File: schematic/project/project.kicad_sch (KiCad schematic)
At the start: 4 parts, among them U1 NFC IC

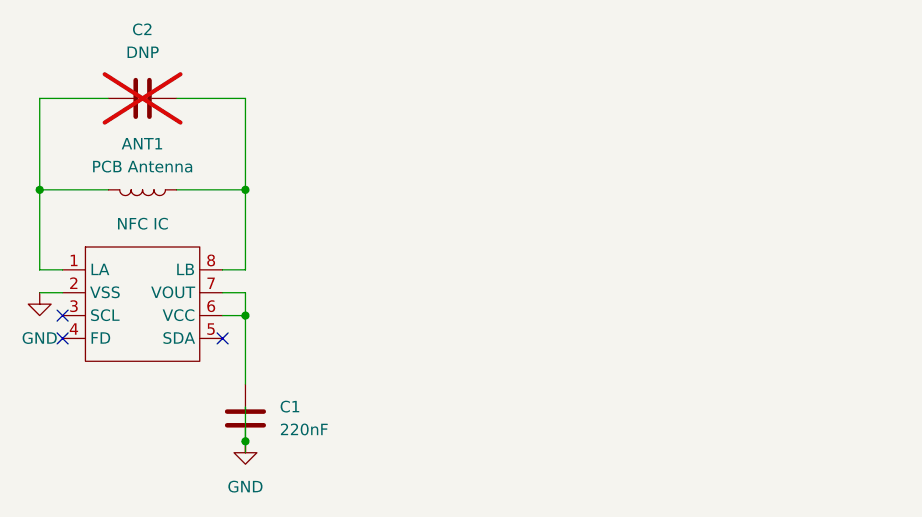
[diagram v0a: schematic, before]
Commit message: ??
After not realizing for nearly two weeks I finally committed proper workfiles with updated progress on the PCB of the card
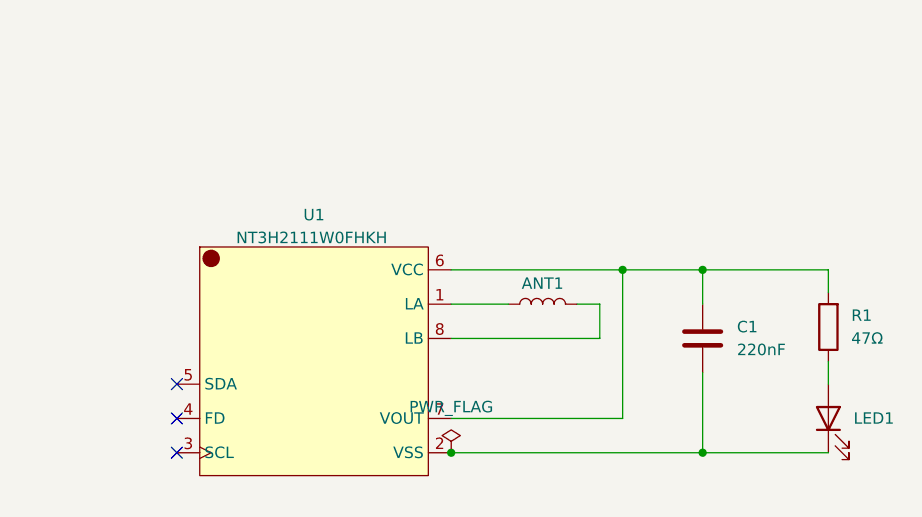
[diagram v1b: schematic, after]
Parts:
- removed C2: DNP, Capacitor_SMD:C_0805_2012Metric, symbol Device:C
- removed U1: NFC IC, Package_SO:TSSOP-8_3x3mm_P0.65mm, symbol local:NT3H2111W0FTTJ
- added LED1: LED, LED_SMD:LED_0805_2012Metric, symbol Device:LED
- added R1: 47Ω, Resistor_SMD:R_0805_2012Metric, symbol Device:R
- added U1: NT3H2111W0FHKH, NT3H2111W0FHKH:QFN8P50_160X160X50L40X20N, symbol NT3H2111W0FKH:NT3H2111W0FHKH
- ANT1: value PCB Antenna -> Class5_Circular_D35mm_ID20mm_8T_W0.56_G0.30; footprint NFC_Antenna:Class4_48x25mm_5T -> Antenna:Class5_Circular_D35mm_ID20mm_8T_W0.56_G0.30; now left out of the parts list
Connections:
- net at ANT1.1: now also U1.1 (LA)
- net at ANT1.2: now also U1.8 (LB)
- net at C1.1: now also R1.2, U1.6 (VCC), U1.7 (VOUT)
- net GND: no longer names the net of C1.2
- net GND: now also LED1.1 (K), U1.2 (VSS)
- new net: LED1.2 (A), R1.1
